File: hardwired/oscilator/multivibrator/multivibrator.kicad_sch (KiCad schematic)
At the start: 19 parts, among them Q1 NPN, Q3 PNP, U1 Opamp_Dual, U2 BUF634P

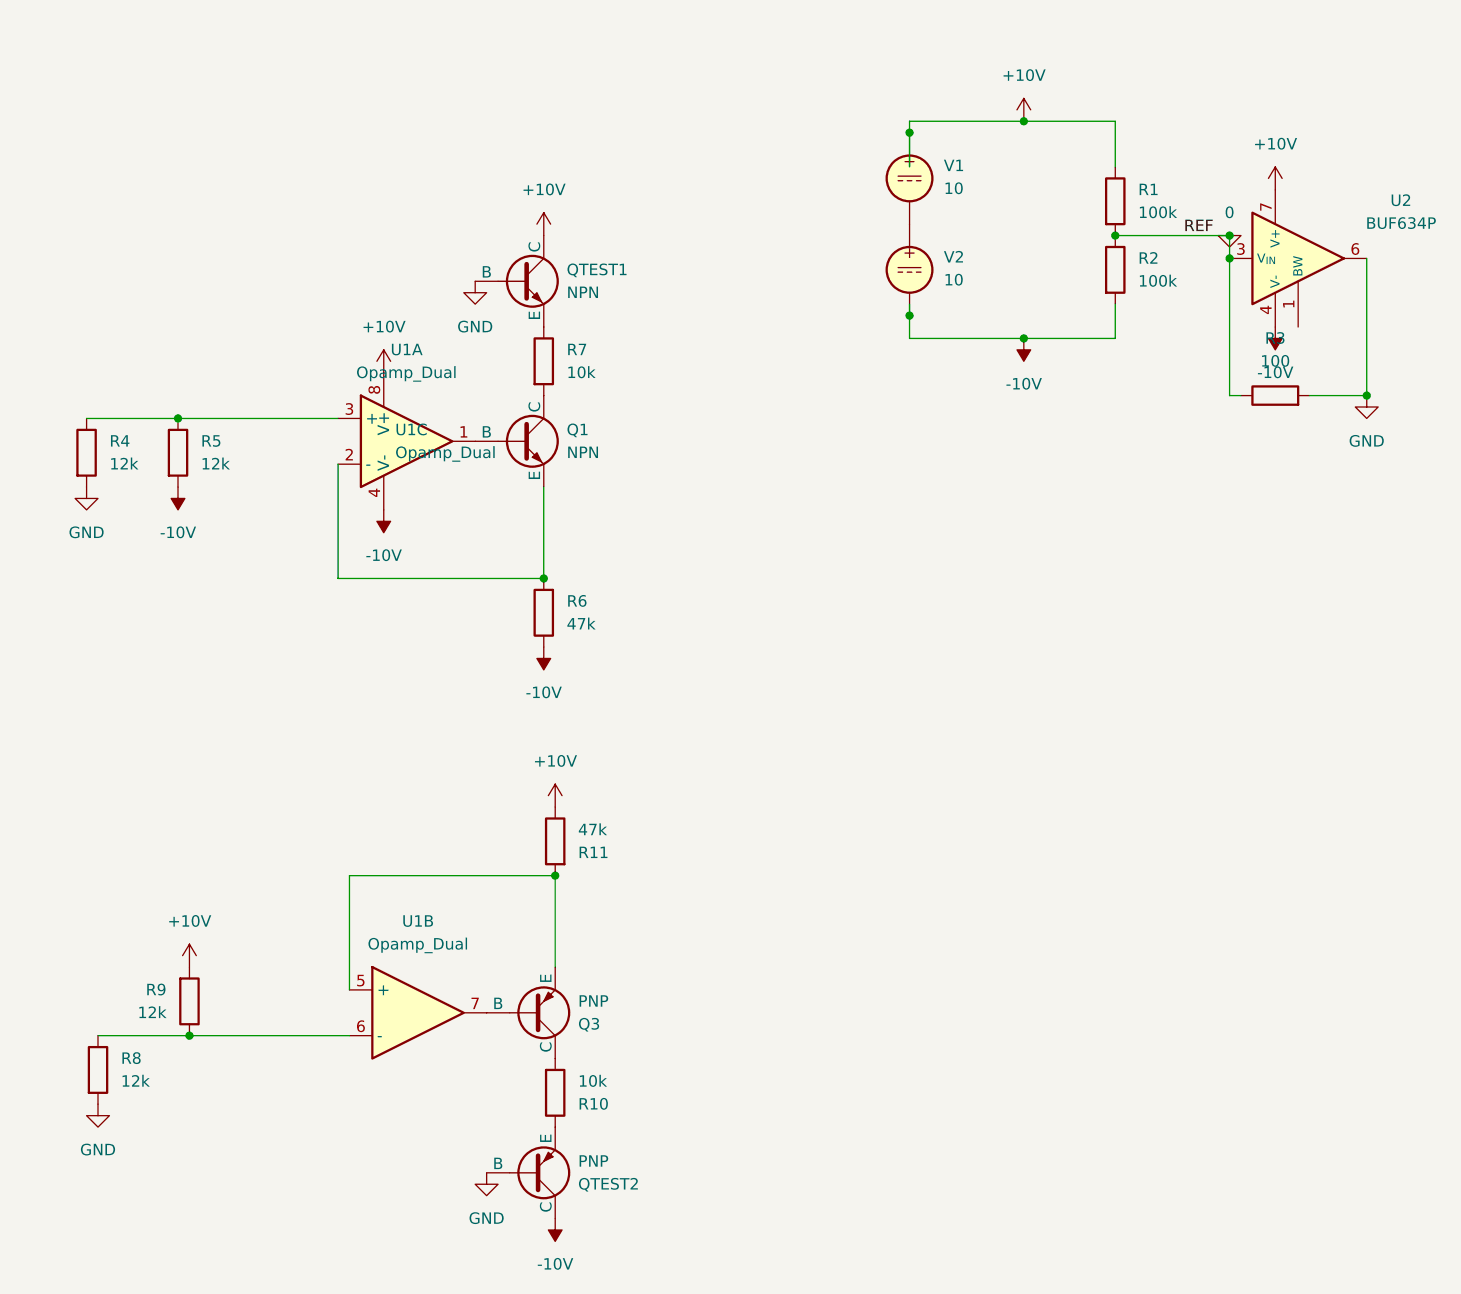
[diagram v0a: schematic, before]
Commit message: A whole bunch of circuits
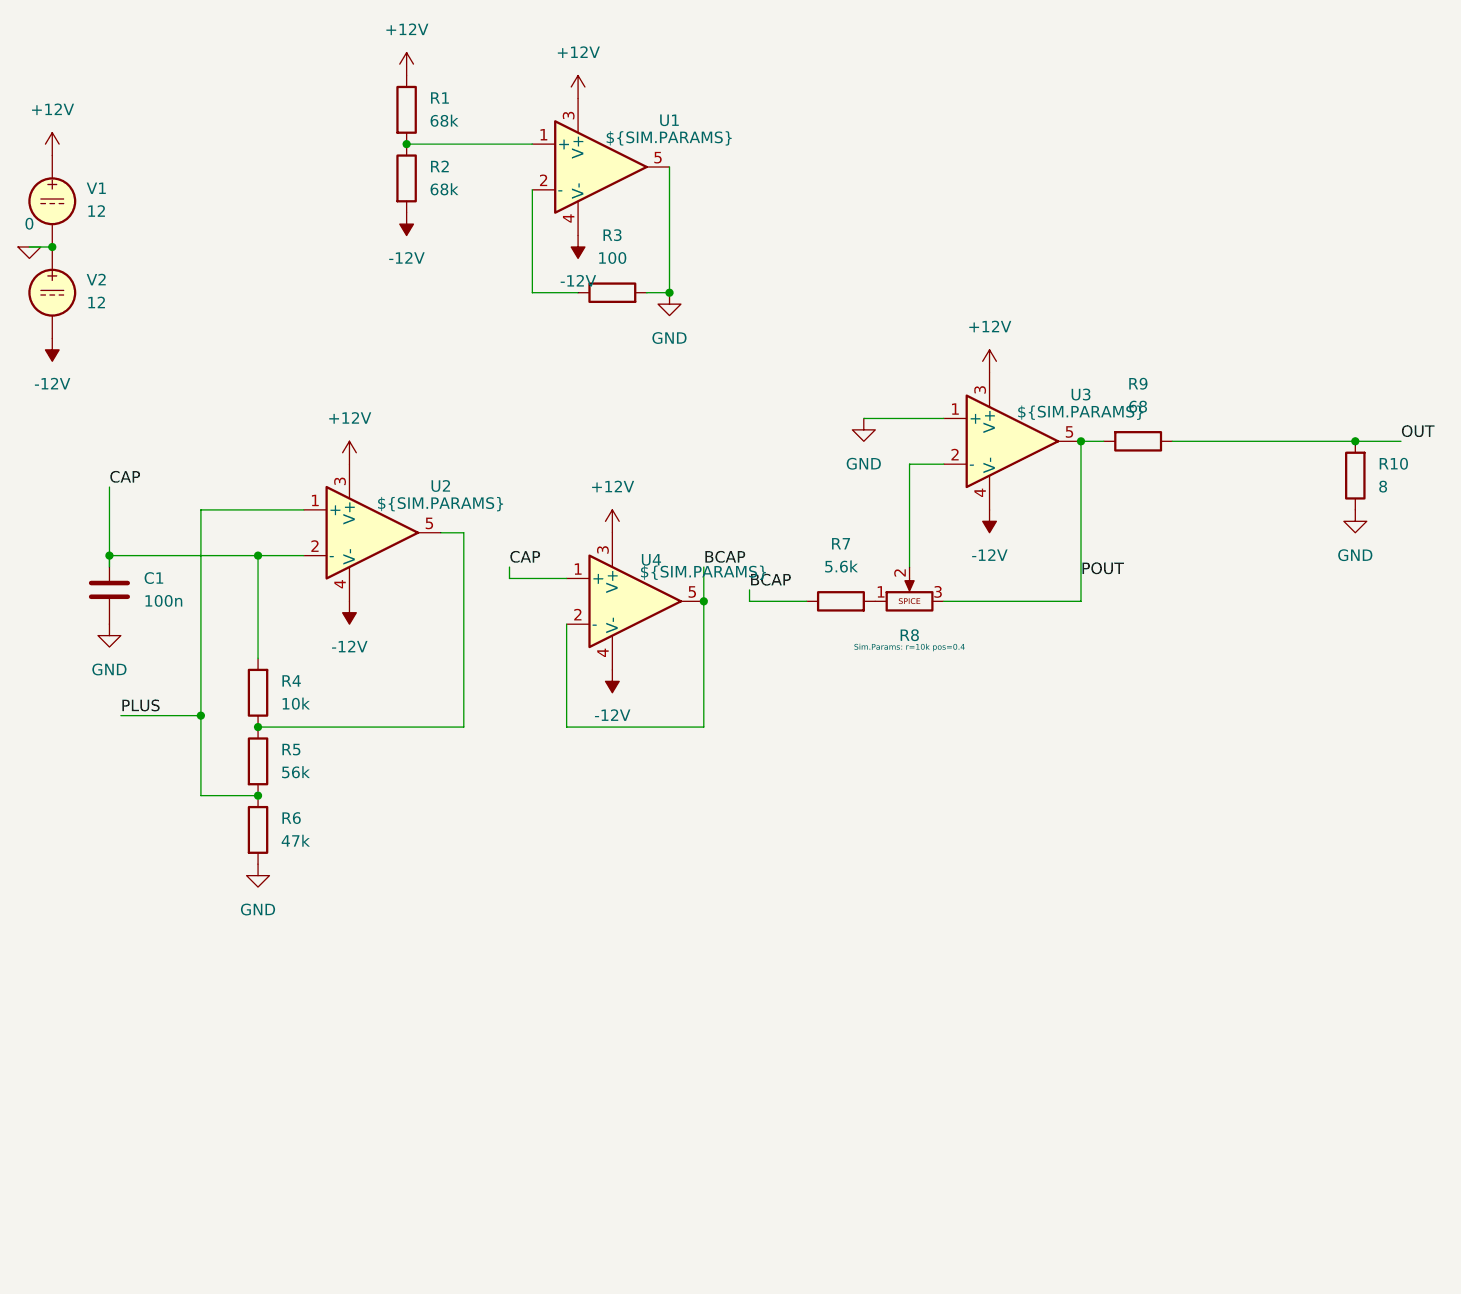
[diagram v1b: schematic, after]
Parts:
- removed Q1, QTEST1: NPN, Connector_PinHeader_2.54mm:PinHeader_1x03_P2.54mm_Vertical, symbol Simulation_SPICE:NPN
- removed Q3, QTEST2: PNP, Connector_PinHeader_2.54mm:PinHeader_1x03_P2.54mm_Vertical, symbol Simulation_SPICE:PNP
- removed R11: 47k, Resistor_THT:R_Axial_DIN0309_L9.0mm_D3.2mm_P12.70mm_Horizontal, symbol Device:R
- removed R8: 12k, Resistor_THT:R_Axial_DIN0309_L9.0mm_D3.2mm_P12.70mm_Horizontal, symbol Device:R
- removed U1: Opamp_Dual, Package_DIP:DIP-8_W7.62mm_Socket, symbol Device:Opamp_Dual
- removed U2: BUF634P, Package_DIP:DIP-8_W7.62mm_Socket, symbol Amplifier_Buffer:BUF634U
- added C1: 100n, symbol Device:C
- added R8: Potentiometer, symbol Simulation_SPICE:Potentiometer
- added U1, U2, U3, U4: ${SIM.PARAMS}, symbol Simulation_SPICE:OPAMP
- R1, R2: value 100k -> 68k; footprint Resistor_THT:R_Axial_DIN0309_L9.0mm_D3.2mm_P12.70mm_Horizontal -> (none)
- R10: value 10k -> 8; footprint Resistor_THT:R_Axial_DIN0309_L9.0mm_D3.2mm_P12.70mm_Horizontal -> (none)
- R3, R6: footprint Resistor_THT:R_Axial_DIN0309_L9.0mm_D3.2mm_P12.70mm_Horizontal -> (none)
- R4: value 12k -> 10k; footprint Resistor_THT:R_Axial_DIN0309_L9.0mm_D3.2mm_P12.70mm_Horizontal -> (none)
- R5: value 12k -> 56k; footprint Resistor_THT:R_Axial_DIN0309_L9.0mm_D3.2mm_P12.70mm_Horizontal -> (none)
- R7: value 10k -> 5.6k; footprint Resistor_THT:R_Axial_DIN0309_L9.0mm_D3.2mm_P12.70mm_Horizontal -> (none)
- R9: value 12k -> 68; footprint Resistor_THT:R_Axial_DIN0309_L9.0mm_D3.2mm_P12.70mm_Horizontal -> (none)
- V1, V2: value 10 -> 12; footprint Connector_PinHeader_2.54mm:PinHeader_1x02_P2.54mm_Horizontal -> (none)
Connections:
- net 0: now also V1.2, V2.1; no longer R1.2, R2.1, R3.1
- net GND: now also R10.1, R6.2, C1.2, U1.5, U3.1 (+); no longer R4.2
- net OUT: now reaches R10.2
- net OUT: now also R9.1
- net at R7.2: now also R8.1
- net BCAP: now reaches R7.1
- net BCAP: now also U4.2 (-), U4.5
- net at R4.1, R5.1: now also U2.5
- net +10V renamed +12V
- net +12V: now also U1.3 (V+), U2.3 (V+), U3.3 (V+), U4.3 (V+); no longer R9.2
- net -10V renamed -12V
- net -12V: now also U1.4 (V-), U2.4 (V-), U3.4 (V-), U4.4 (V-); no longer R5.2, R6.1
- new net: R3.1, U1.2 (-)
- new net: R8.2, U3.2 (-)
- new net: R1.2, R2.1, U1.1 (+)
- new net CAP: C1.1, R4.2, U2.2 (-), U4.1 (+)
- new net PLUS: R5.2, R6.1, U2.1 (+)
- new net POUT: R8.3, R9.2, U3.5
